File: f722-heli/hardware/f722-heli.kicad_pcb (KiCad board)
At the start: 6 copper layers, 39.2 x 25.4 mm, 156 parts, among them J1 USB4105-GF-A-120, J10 PORT B / JST GH, J11 PORT C / JST GH, J12 DSM / JST ZH, J2 S1 / GND-VX-S, J3 S2 / GND-VX-S, J4 S3 / GND-VX-S, J5 TAIL / GND-VX-S, J6 ESC / GND-VX-S, J7 RPM / GND-VX-S, J8 SBUS / GND-VX-S, J9 PORT A / JST GH, Q1 BSS138LT1G, Q2 BSS138LT1G, SW1 BOOT / KMT031NGJLHS, U1 STM32F722RET6, U10 TPS2553DRVR / USB input limit, U11 TPS2553DRVR / DSM output limit, U12 USBLC6-4SC6 / header clamp, U13 USBLC6-4SC6 / header clamp, U14 TPD4E05U06DQAR / UART ESD, U15 TPD4E05U06DQAR / UART ESD, U16 PESD15VS2UT,215 / 15V ESD, U2 ICM-42688-P, U3 W25N01GVZEIG / 128MiB, U4 DPS368XTSA1 / 0x76, U5 TPS259472ARPWR, U6 TPS63070RNMR / nominal 5.088V, U7 TPS2117DRLR / ABC priority mux, U8 TPS2121RUXR / BEC-priority co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, U9 TPS62162DSGR / 3.3V 1A, Y1 8MHz / CL10pF / TAXM8M4RDBCCT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

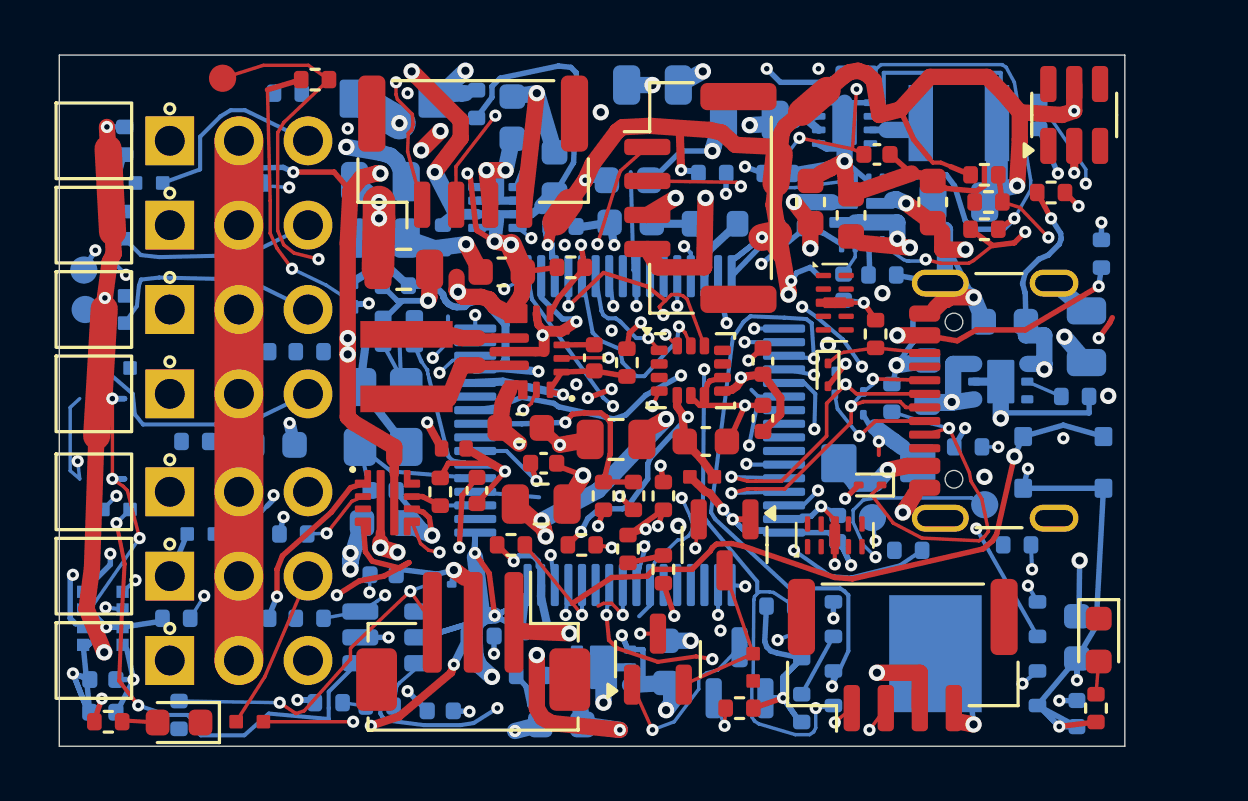
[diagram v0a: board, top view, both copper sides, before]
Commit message: F722: add final routed PCB and paired schematics
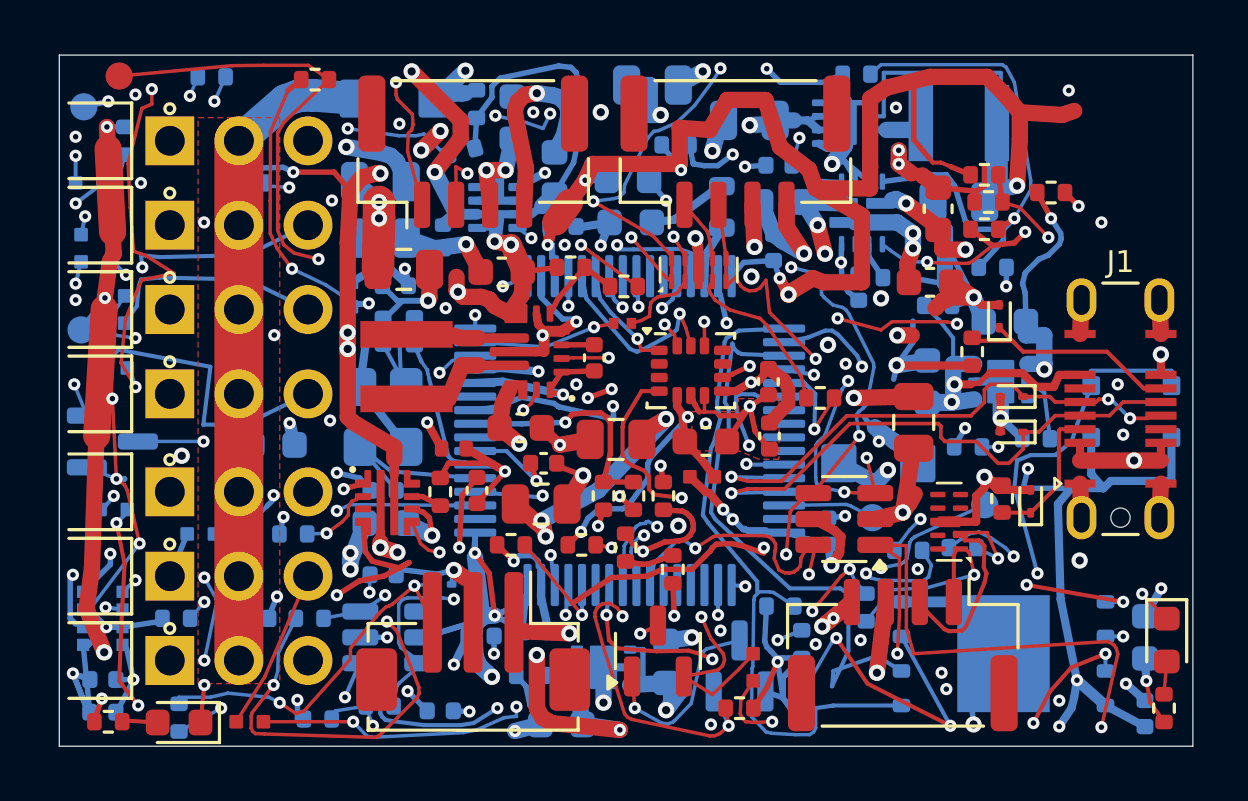
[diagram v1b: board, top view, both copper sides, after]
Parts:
- C63, C65, Q2: moved to B.Cu
- C75, D3, D4, R14, R32: moved to F.Cu
- J1: value USB4105-GF-A-120 -> USB4145-03-0170-C; footprint F722_Heli:USB_C_Receptacle_GCT_USB4105-xx-A_16P_TopMnt_Horizontal -> F722_Heli:USB_C_Receptacle_GCT_USB4145-03-0170-C_16P_Vertical
- J2, J3, J4, J5, J6, J7, J8: footprint F722_Heli:Samtec_HTSW-101-08-L-T-RA_TripleRow -> F722_Heli:Samtec_HTSW-101-08-L-T-RA_TripleRow_OpenEdgeSilk
- R16: value 0.15R / 1% / VCAP ESR -> 0.12R / 1% / VCAP ESR; footprint F722_Heli:R_0603_1608Metric -> F722_Heli:R_Panasonic_ERJ3R_0603
- R31: footprint F722_Heli:R_0402_1005Metric -> F722_YAGEO:R_0201_0603Metric_YAGEO_AC; moved to F.Cu
- R5: footprint F722_Heli:R_0402_1005Metric -> F722_Heli:R_0402_1005Metric_R5_ClearPin1Silk
- moved R35 28.5 mm to (33.2, 18.1), turned to 180 degrees
- moved R34 24.3 mm to (29.6, 20.3), turned to 90 degrees
- moved Q2 22.8 mm to (1.95, 14.2), turned to 0 degrees
- moved R56 21.3 mm to (14.8, 3.55), turned to -165 degrees
- moved U12 17.1 mm to (28.9, 17.1), turned to 180 degrees
- moved R31 14.9 mm to (20.7, 9.86), turned to 180 degrees
- moved R30 10.7 mm to (5.60, 0.80), turned to 180 degrees
- moved R32 9.03 mm to (28.0, 12.6)
- moved R61 8.62 mm to (34.3, 7.80)
- moved C75 7.09 mm to (31.4, 13.5), turned to -90 degrees
- moved D6 6.66 mm to (34.5, 9.60), turned to 90 degrees
- moved D4 6.52 mm to (35.0, 12.6), turned to 180 degrees
- moved R69 6.29 mm to (32.3, 9.20), turned to 0 degrees
- moved TP4 6.00 mm to (0.90, 1.90)
- moved D5 5.93 mm to (35.7, 16.4), turned to 90 degrees
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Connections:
- U14 pad 10: unconnected-(U14-NC10-Pad10) -> PORT_A_RX_EXT
- U14 pad 6: unconnected-(U14-NC6-Pad6) -> PORT_B_TX_EXT
- U14 pad 7: unconnected-(U14-NC7-Pad7) -> PORT_B_RX_EXT
- U14 pad 9: unconnected-(U14-NC9-Pad9) -> PORT_A_TX_EXT
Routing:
- net SERVO1_MCU: track 3.09 -> 101.0 mm, vias 1 -> 5
- net TAIL_MCU: track 5.30 -> 101.6 mm, vias 1 -> 7
- net SERVO2_MCU: track 3.64 -> 99.0 mm, vias 1 -> 9
- net SERVO3_MCU: track 5.31 -> 59.1 mm, vias 1 -> 5
- net PORT_A_RX_EXT: track 4.87 -> 52.5 mm, vias 1 -> 5
- net LED_RED_K: track 2.36 -> 42.2 mm, vias 0 -> 5
- net PORT_C_TX_MCU: track 6.93 -> 45.9 mm, vias 1 -> 4
- net SBUS_HV: track 6.03 -> 39.7 mm, vias 0 -> 4
- net RPM_LV: track 1.74 -> 34.8 mm, vias 1 -> 4
- net ABC_PG: track 59.6 -> 27.4 mm, vias 7 -> 5
- net +5V_BEC: track 62.0 -> 32.7 mm, vias 7 -> 5
- net SBUS_LV: track 1.93 -> 26.6 mm, vias 1 -> 2
- net DSM_RX_MCU: track 29.6 -> 53.2 mm, vias 3 -> 5
- net LED_GREEN_K: track 0.96 -> 23.9 mm, vias 0 -> 2
- net +5V_PERIPH: track 22.0 -> 44.0 mm, vias 7 -> 8
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- added copper zone on F.Cu, net GND
- added copper zone on F.Cu, net VX_RAW
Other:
- board size 39.2 x 25.4 mm -> 41.7 x 25.4 mm
